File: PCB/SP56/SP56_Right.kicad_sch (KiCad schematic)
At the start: 95 parts, among them J101 USB_C_Receptacle_USB2.0, J103 Conn_01x01_Female, J104 Conn_01x01_Female, J106 SM02B-SRSS-TB(LF)(SN), Q102 A03407, SW101 SW_PUSH, SW102 SW_PUSH, SW103 SW_PUSH, SW104 SW_PUSH, SW105 SW_PUSH, SW106 SW_PUSH, SW107 SW_PUSH, SW108 SW_PUSH, SW109 SW_PUSH, SW110 SW_PUSH, SW111 SW_PUSH, SW112 SW_PUSH, SW113 SW_PUSH, SW114 SW_PUSH, SW115 SW_PUSH, SW116 SW_PUSH, SW117 SW_PUSH, SW118 SW_PUSH, SW119 SW_PUSH, SW120 SW_PUSH, SW121 SW_PUSH, SW122 SW_PUSH, SW123 SW_PUSH, SW124 SW_PUSH, SW125 Rotary_Encoder_Switch, SW126 SW_PUSH, SW127 SW_PUSH, SW128 SW_PUSH, U101 LN2054Y42AMR, U102 E73-2G4M08S1C, U103 AP2112K-3.3, Y101 32.768kHz

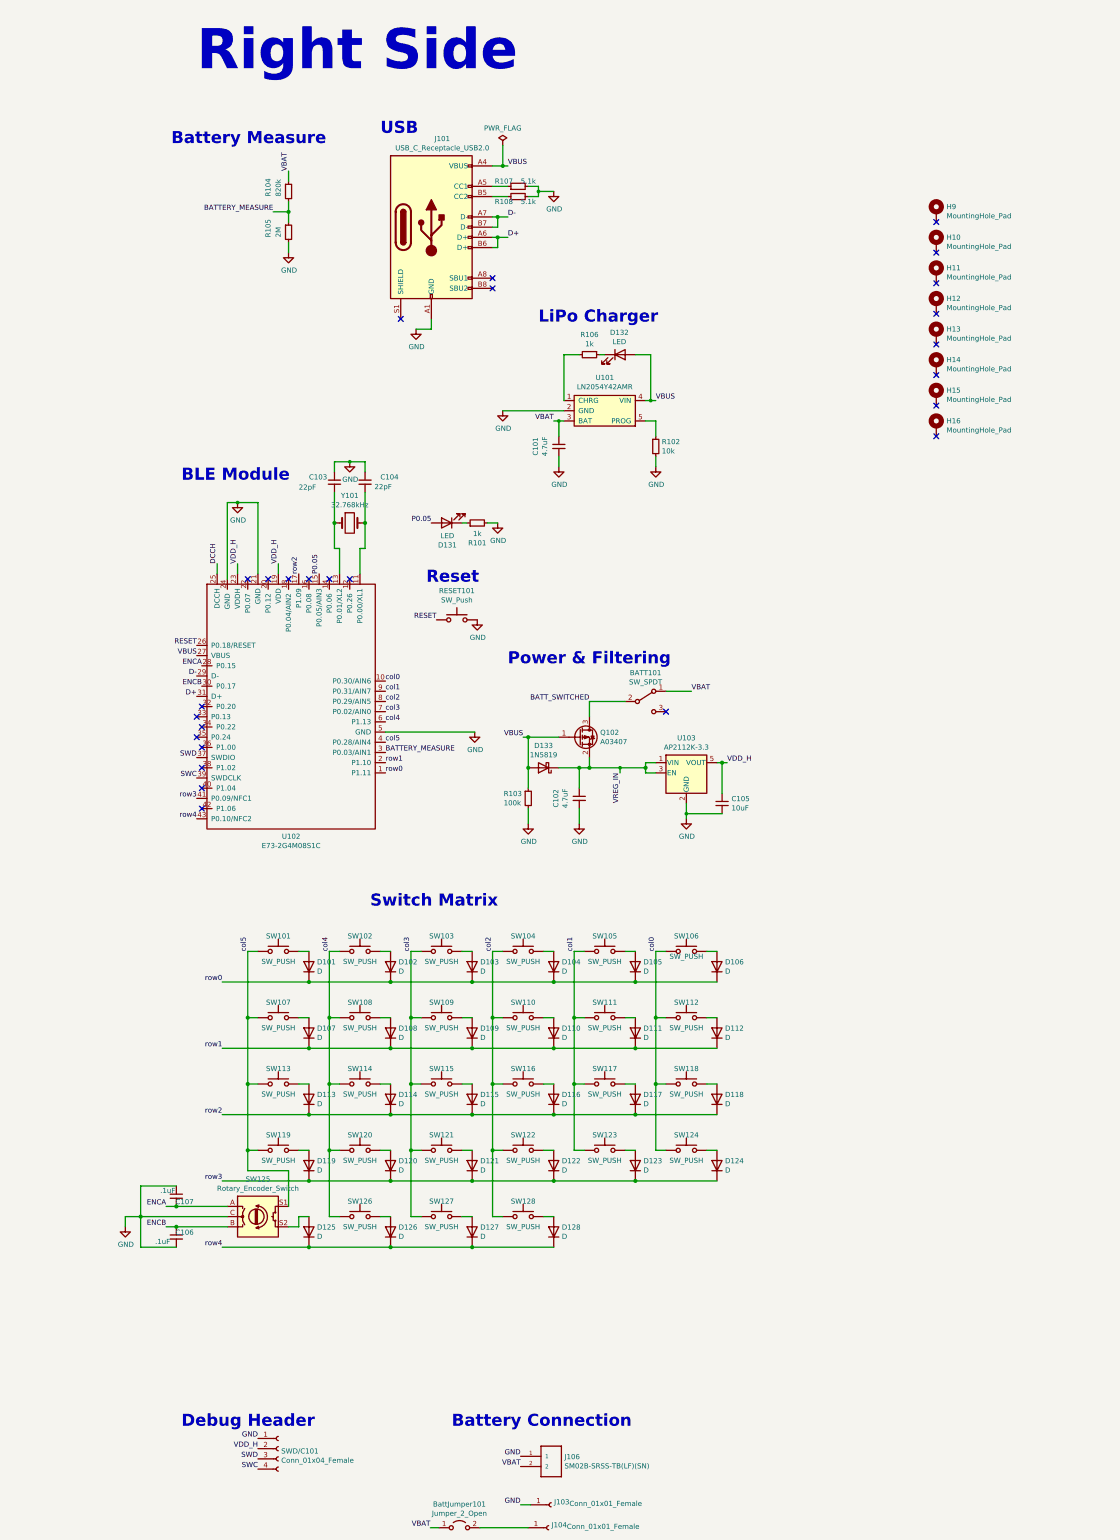
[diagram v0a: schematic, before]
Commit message: ready for jlc quote
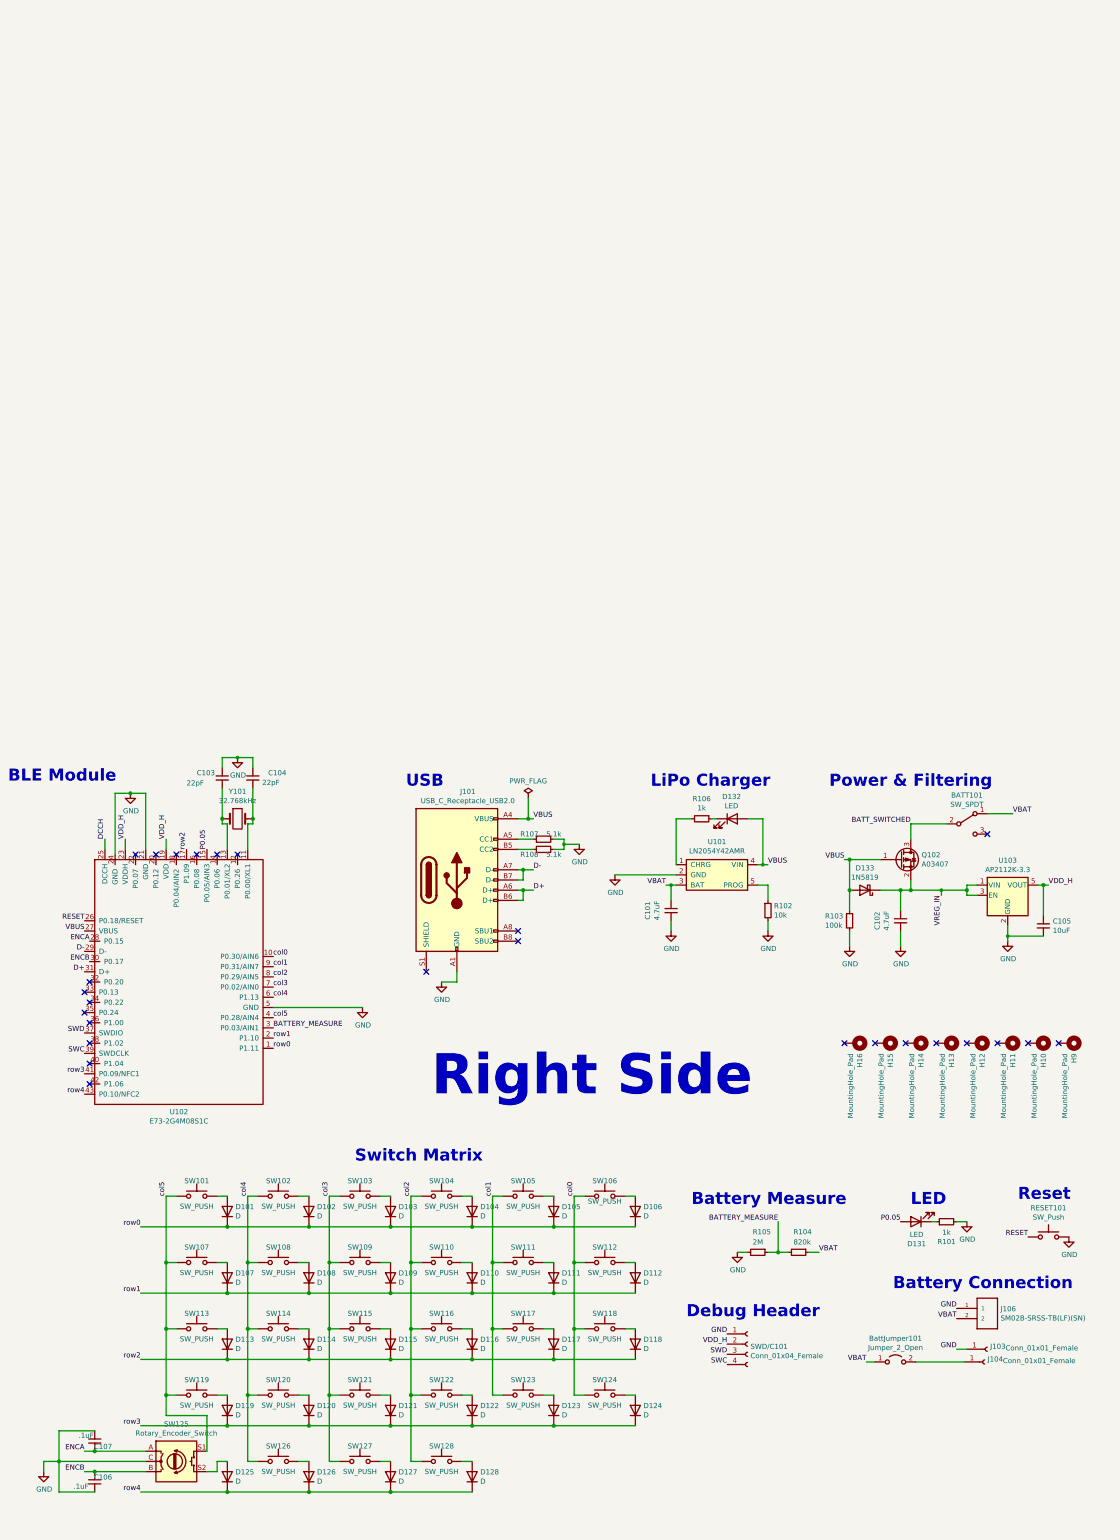
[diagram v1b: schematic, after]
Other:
- note added: "LED"
- company: (none) -> CO Boards
- title: (none) -> SP56
- moved on the sheet: BATT101, BattJumper101, C101, C102, C103, C104, C105, C106, C107, D101, D102, D103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
